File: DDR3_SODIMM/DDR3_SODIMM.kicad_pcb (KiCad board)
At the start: 2 copper layers, 67.8 x 30.1 mm, 1 part, among them U1 DDR3_SODIMM_PINOUT

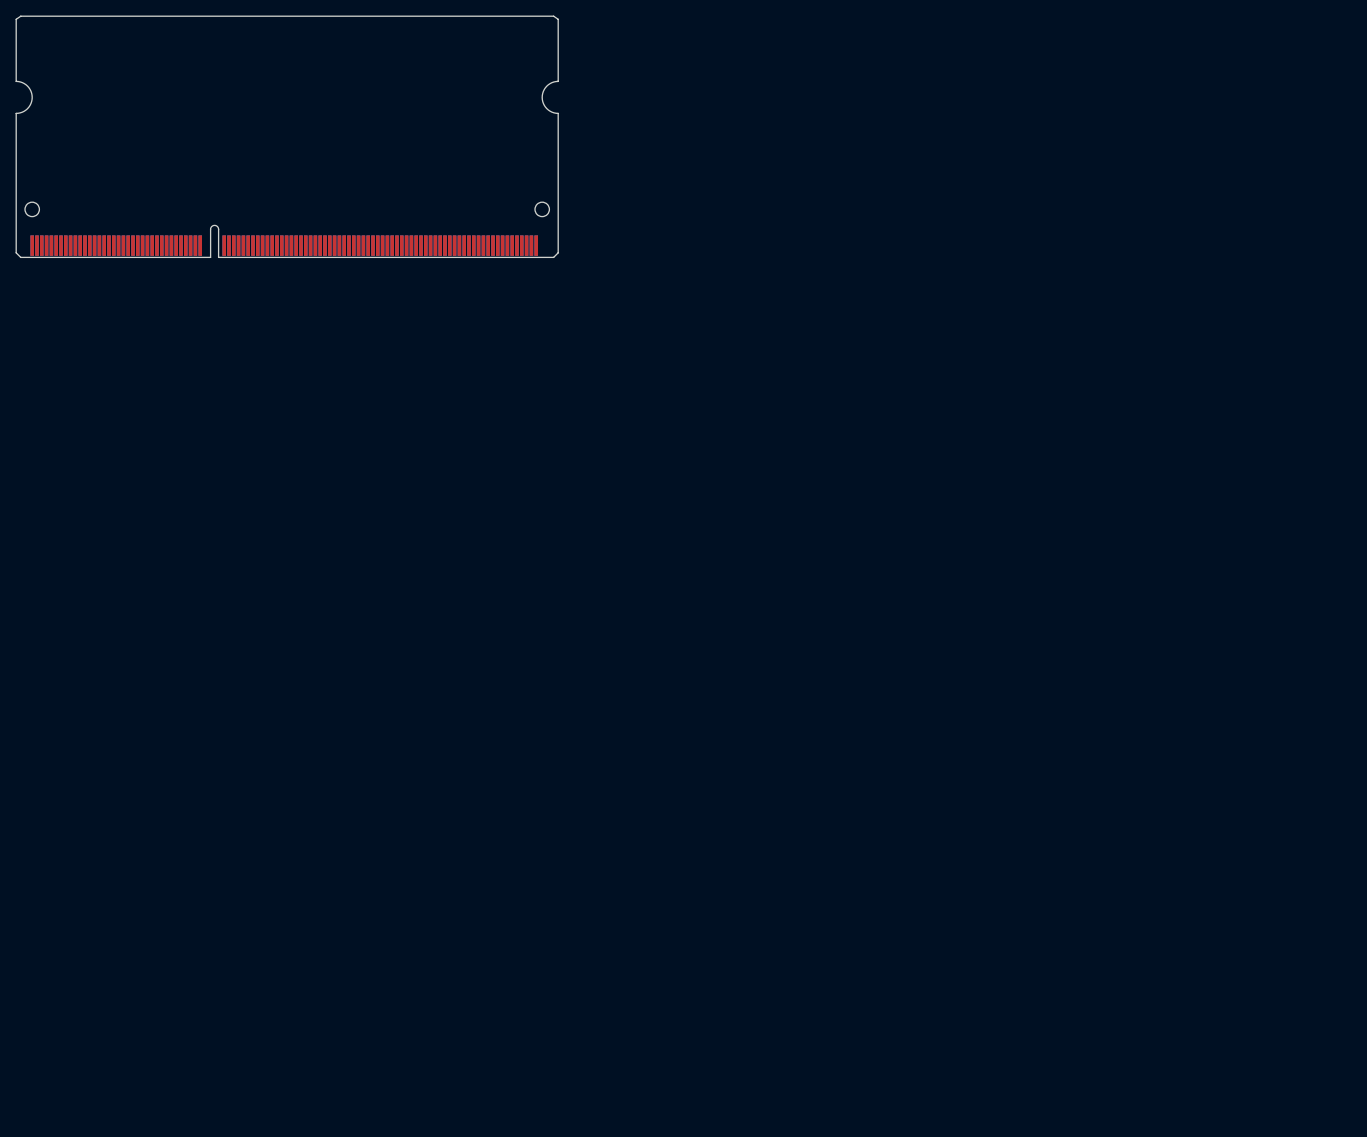
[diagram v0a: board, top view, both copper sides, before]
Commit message: ddr4 sodimm
This is the first trying
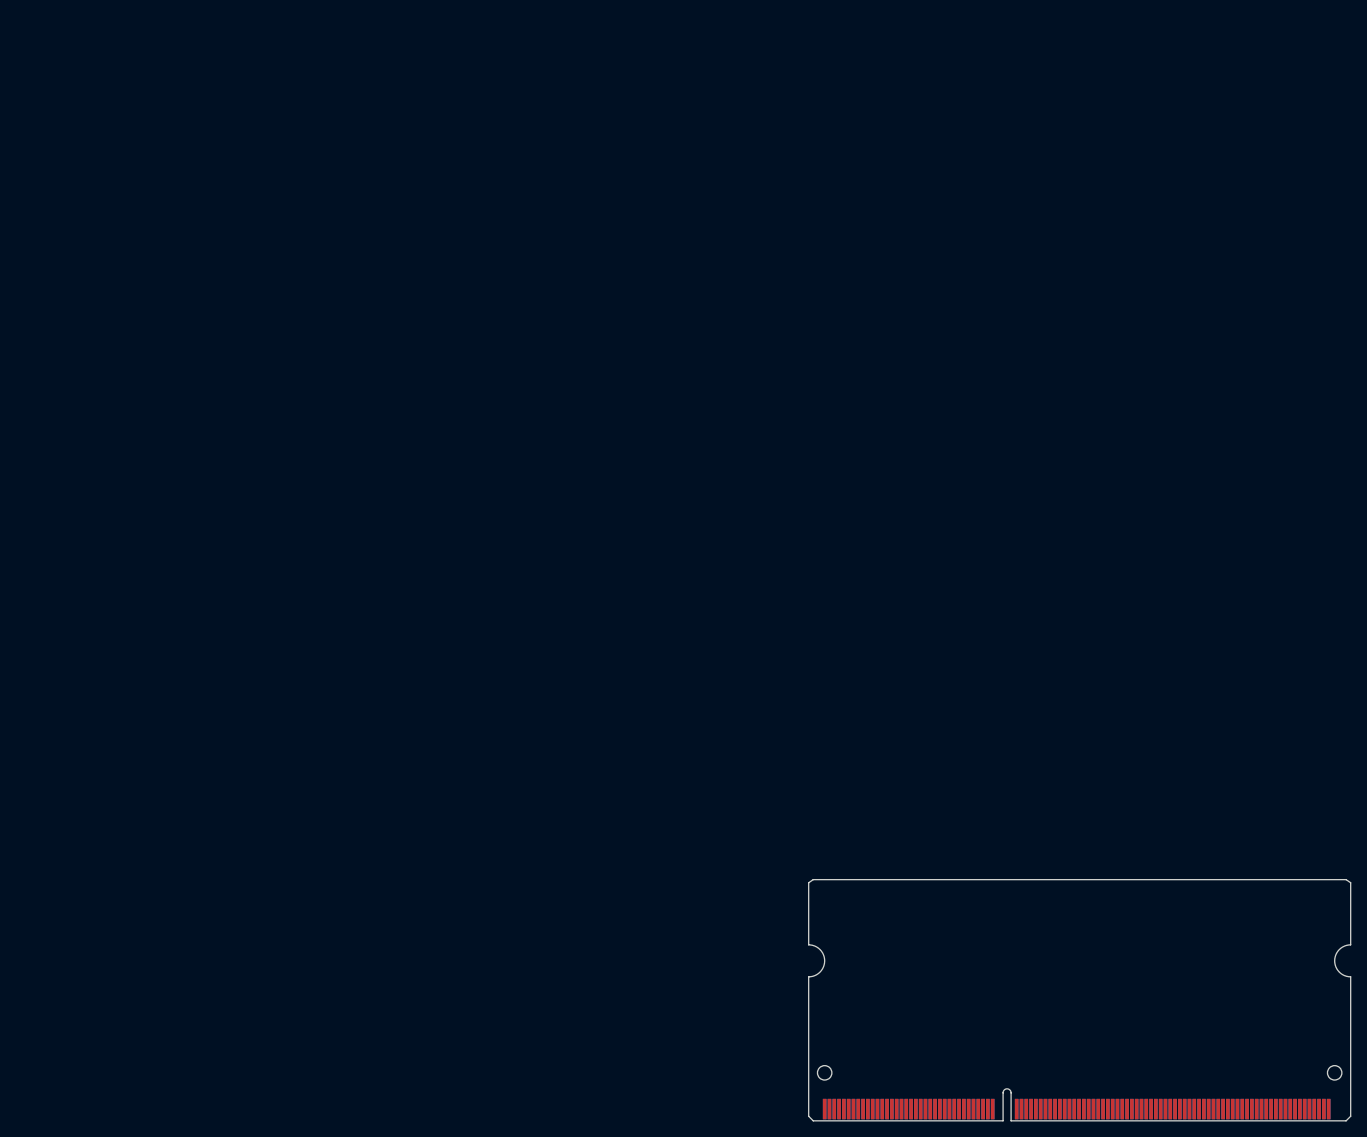
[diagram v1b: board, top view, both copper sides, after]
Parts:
- moved U1 146.5 mm to (101.1, 107.0)
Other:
- board size 67.8 x 30.1 mm -> 67.8 x 30.2 mm
- net class Default removed
